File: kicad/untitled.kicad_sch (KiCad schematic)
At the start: 16 parts, among them J2 NMJ4HCD2, J3 AudioJack3_Dual_Switch, J4 AudioJack3_Dual_Switch, J5 NMJ4HCD2, SW5 SW_Slide_DPDT, U2 OPA1678

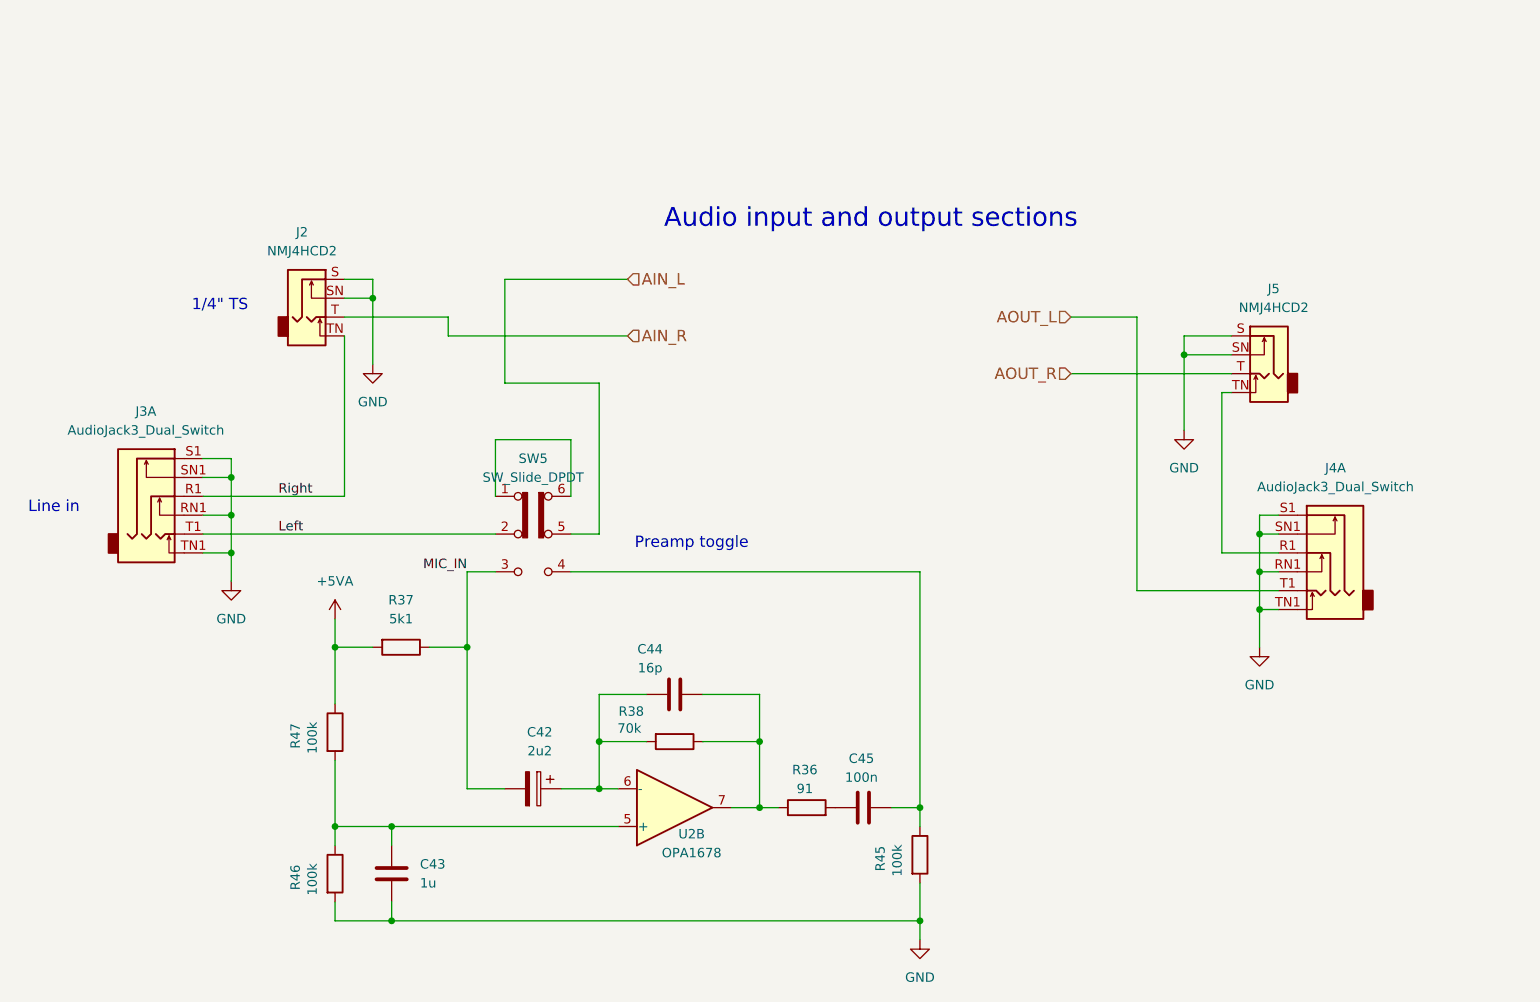
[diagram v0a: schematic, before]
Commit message: aaa
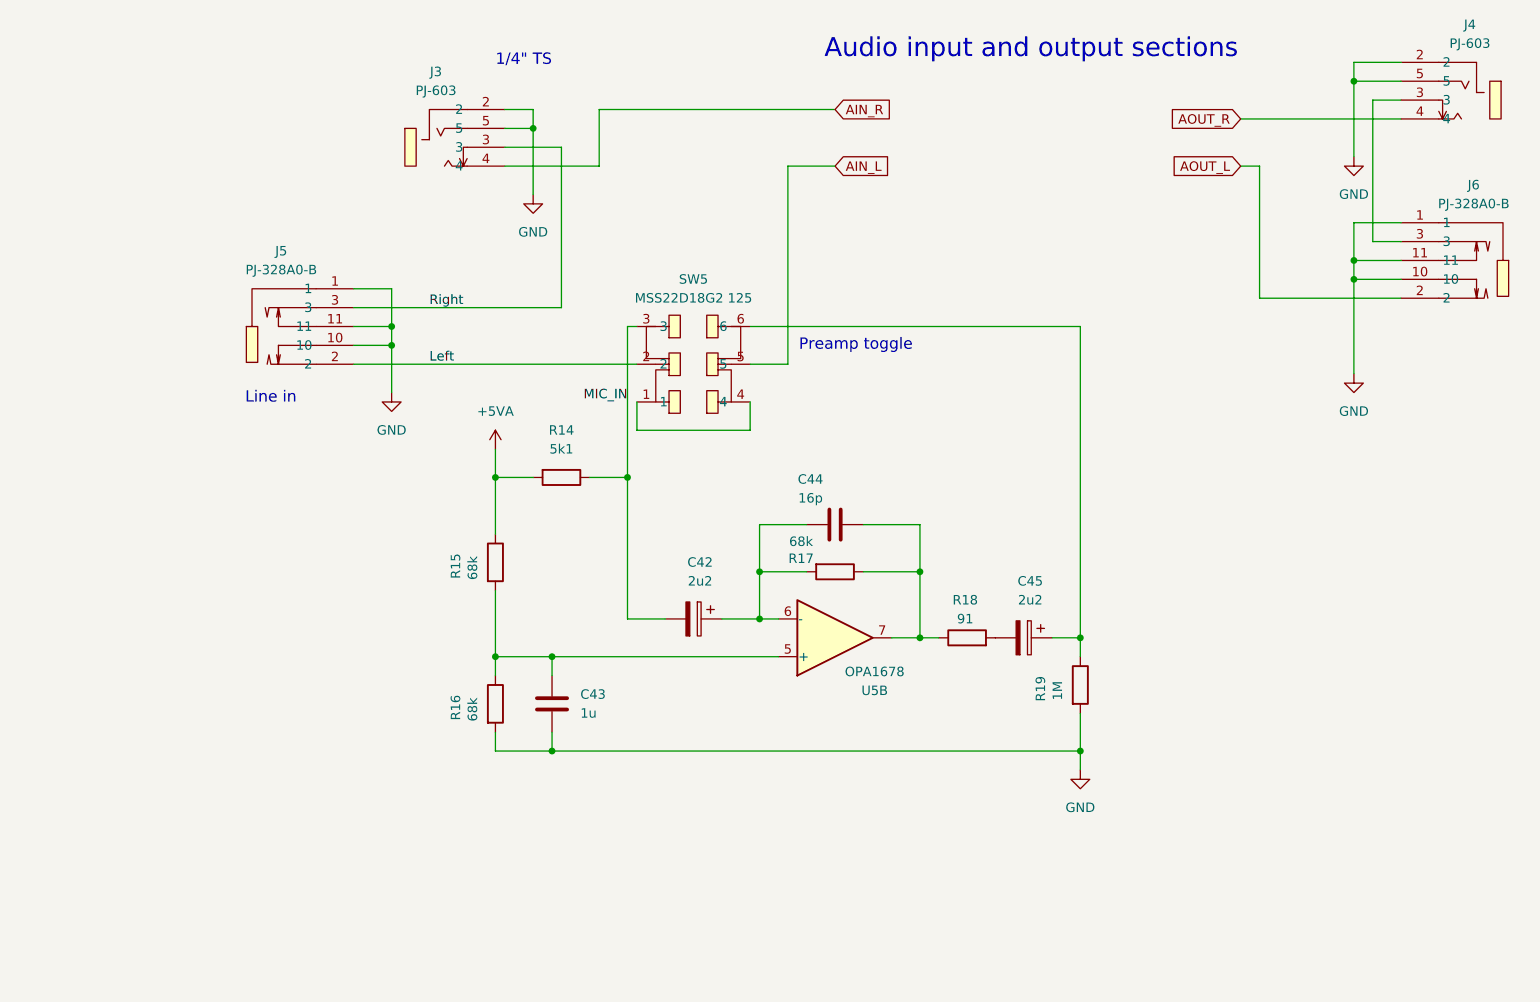
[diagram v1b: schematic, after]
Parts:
- removed C45: 100n, symbol Device:C
- removed J2, J5: NMJ4HCD2, Connector_Audio:Jack_6.35mm_Neutrik_NMJ4HCD2_Horizontal, symbol Connector_Audio:NMJ4HCD2
- removed J3, J4: AudioJack3_Dual_Switch, symbol Connector_Audio:AudioJack3_Dual_Switch
- removed R36: 91, symbol Device:R
- removed R37: 5k1, symbol Device:R
- removed R38: 70k, symbol Device:R
- removed R45, R46, R47: 100k, symbol Device:R
- removed SW5: SW_Slide_DPDT, symbol Switch:SW_Slide_DPDT
- removed U2: OPA1678, Package_SO:SOIC-8_3.9x4.9mm_P1.27mm, symbol Amplifier_Operational:NE5532
- added C45: 2u2, Capacitor_SMD:CP_Elec_4x5.4, symbol Device:C_Polarized
- added J3, J4: PJ-603, easyeda2kicad:AUDIO-TH_PJ-603, symbol easyeda2kicad:PJ-603
- added J5, J6: PJ-328A0-B, easyeda2kicad:AUDIO-TH_PJ-328A0-B, symbol easyeda2kicad:PJ-328A0-B
- added R14: 5k1, Resistor_SMD:R_0402_1005Metric, symbol Device:R
- added R15, R16, R17: 68k, Resistor_SMD:R_0402_1005Metric, symbol Device:R
- added R18: 91, Resistor_SMD:R_0402_1005Metric, symbol Device:R
- added R19: 1M, Resistor_SMD:R_0402_1005Metric, symbol Device:R
- added SW5: MSS22D18G2 125, easyeda2kicad:SW-TH_SHOU_MSS22D18G2, symbol easyeda2kicad:MSS22D18G2125
- added U5: OPA1678, Package_SO:SOIC-8_3.9x4.9mm_P1.27mm, symbol Amplifier_Operational:OPA1678
- C42: footprint (none) -> Capacitor_SMD:CP_Elec_4x5.4
- C43, C44: footprint (none) -> Capacitor_SMD:C_0402_1005Metric
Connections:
- net +5VA: now also R14.2, R15.1
- net AIN_L: now also SW5.5
- net AIN_R: now also J3.4
- net AOUT_L: now also J6.2
- net AOUT_R: now also J4.4
- net GND: now also J3.2, J3.5, J4.2, J4.5, J5.1, J5.10, J5.11, J6.1, J6.10, J6.11, R16.2, R19.2
- net Left: now also J5.2, SW5.2
- net MIC_IN: now also R14.1, SW5.3
- net Right: now also J3.3, J5.3
- net at C43.1: now also R15.2, R16.1, U5.5 (+)
- net at C42.1, C44.1: now also R17.2, U5.6 (-)
- net at C44.2: now also R17.1, R18.1, U5.7
- new net: J4.3, J6.3
- new net: C45.1, R19.1, SW5.6
- new net: C45.2, R18.2
- new net: SW5.1, SW5.4
